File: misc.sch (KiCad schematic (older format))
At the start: 38 parts, among them J13 MICROSD_SLOT_TFP09-2-12B, P13 EXT_SD, P14 LCD, P15 LIMIT_SWITCHES, P16 LIMIT_SWITCHES_V, P17 CONN_01X03, P18 CONN_01X03, P19 CONN_01X03, P20 CONN_01X03, P21 THERMISTORS, P22 CONN_01X05, SW1 RESET, U2 24LC256

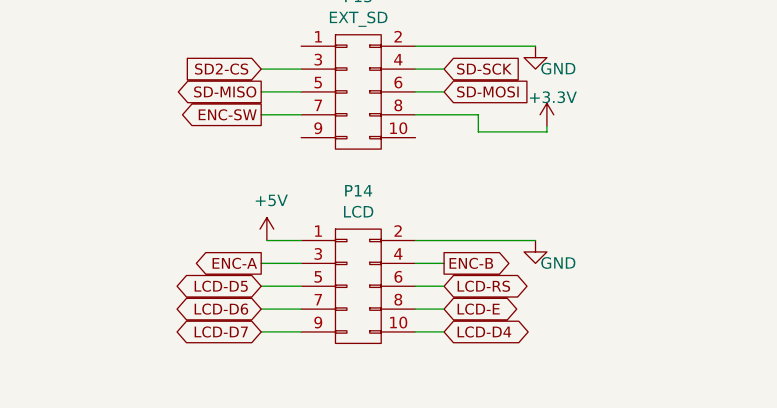
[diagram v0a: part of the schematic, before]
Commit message: More 3d stuff
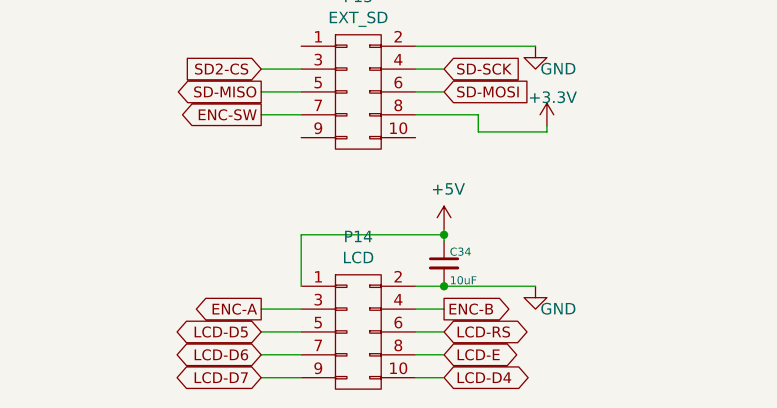
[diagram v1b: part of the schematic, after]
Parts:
- added C34: 10uF, Capacitors_SMD:C_0805, symbol C_Small
- P22: footprint geda-footprints:CON_HDR_1x5 -> armin-footprints:CON_HDR_1x5_2.54mm
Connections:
- net +5V: now also C34.1
- net GND: now also C34.2
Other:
- moved on the sheet: P14
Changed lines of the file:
@@
 SD-SCK
 $Comp
-L +3.3V #PWR083
+L +3.3V #PWR63
 U 1 1 568CFFAF
 P 1825 1775
-F 0 "#PWR083" H 1825 1625 50  0001 C CNN
+F 0 "#PWR63" H 1825 1625 50  0001 C CNN
 F 1 "+3.3V" H 1825 1925 35  0000 C CNN
 F 2 "" H 1825 1775 50  0000 C CNN
@@
 $EndComp
 $Comp
-L GND #PWR084
+L GND #PWR64
 U 1 1 568C59D5
 P 1825 1975
-F 0 "#PWR084" H 1825 1725 50  0001 C CNN
+F 0 "#PWR64" H 1825 1725 50  0001 C CNN
 F 1 "GND" H 1825 1825 35  0000 C CNN
 F 2 "" H 1825 1975 50  0000 C CNN
@@
 $EndComp
 $Comp
-L GND #PWR085
+L GND #PWR82
 U 1 1 568D834C
 P 9950 2075
-F 0 "#PWR085" H 9950 1825 50  0001 C CNN
+F 0 "#PWR82" H 9950 1825 50  0001 C CNN
 F 1 "GND" H 9958 1901 50  0000 C CNN
 F 2 "" H 9950 2075 50  0000 C CNN
@@
 $EndComp
 $Comp
-L GND #PWR086
+L GND #PWR81
 U 1 1 568D94E5
 P 8825 2325
-F 0 "#PWR086" H 8825 2075 50  0001 C CNN
+F 0 "#PWR81" H 8825 2075 50  0001 C CNN
 F 1 "GND" H 8833 2151 50  0000 C CNN
 F 2 "" H 8825 2325 50  0000 C CNN
@@
 $EndComp
 $Comp
-L +3V3 #PWR087
+L +3V3 #PWR80
 U 1 1 568D9512
 P 8825 1325
-F 0 "#PWR087" H 8825 1175 50  0001 C CNN
+F 0 "#PWR80" H 8825 1175 50  0001 C CNN
 F 1 "+3V3" H 8843 1499 50  0000 C CNN
 F 2 "" H 8825 1325 50  0000 C CNN
@@
 F 0 "P22" H 10527 1838 50  0000 L CNN
 F 1 "CONN_01X05" H 10527 1746 50  0000 L CNN
-F 2 "geda-footprints:CON_HDR_1x5" H 10450 1800 50  0001 C CNN
+F 2 "armin-footprints:CON_HDR_1x5_2.54mm" H 10450 1800 50  0001 C CNN
 F 3 "" H 10450 1800 50  0000 C CNN
 	1    10450 1800
@@
 $EndComp
 $Comp
-L +3V3 #PWR088
+L +3V3 #PWR83
 U 1 1 568D9A56
 P 10250 1525
-F 0 "#PWR088" H 10250 1375 50  0001 C CNN
+F 0 "#PWR83" H 10250 1375 50  0001 C CNN
 F 1 "+3V3" H 10268 1699 50  0000 C CNN
 F 2 "" H 10250 1525 50  0000 C CNN
@@
 $EndComp
 $Comp
-L GND #PWR089
+L GND #PWR67
 U 1 1 568DA443
 P 2875 3725
-F 0 "#PWR089" H 2875 3475 50  0001 C CNN
+F 0 "#PWR67" H 2875 3475 50  0001 C CNN
 F 1 "GND" H 2875 3575 50  0000 C CNN
 F 2 "" H 2875 3725 50  0000 C CNN
@@
 $EndComp
 $Comp
-L GND #PWR090
+L GND #PWR62
 U 1 1 568DA52A
 P 1775 4325
-F 0 "#PWR090" H 1775 4075 50  0001 C CNN
+F 0 "#PWR62" H 1775 4075 50  0001 C CNN
 F 1 "GND" H 1783 4151 50  0000 C CNN
 F 2 "" H 1775 4325 50  0000 C CNN
@@
 $EndComp
 $Comp
-L +3.3V #PWR091
+L +3.3V #PWR65
 U 1 1 568DA65A
 P 2175 3275
-F 0 "#PWR091" H 2175 3125 50  0001 C CNN
+F 0 "#PWR65" H 2175 3125 50  0001 C CNN
 F 1 "+3.3V" H 2193 3449 50  0000 C CNN
 F 2 "" H 2175 3275 50  0000 C CNN
@@
 $EndComp
 $Comp
-L GND #PWR092
+L GND #PWR76
 U 1 1 568D90A7
 P 6475 2225
-F 0 "#PWR092" H 6475 1975 50  0001 C CNN
+F 0 "#PWR76" H 6475 1975 50  0001 C CNN
 F 1 "GND" H 6483 2051 50  0000 C CNN
 F 2 "" H 6475 2225 50  0000 C CNN
@@
 $EndComp
 $Comp
-L +3.3V #PWR093
+L +3.3V #PWR77
 U 1 1 568D9133
 P 6900 1400
-F 0 "#PWR093" H 6900 1250 50  0001 C CNN
+F 0 "#PWR77" H 6900 1250 50  0001 C CNN
 F 1 "+3.3V" H 6918 1574 50  0000 C CNN
 F 2 "" H 6900 1400 50  0000 C CNN
@@
 $EndComp
 $Comp
-L GND #PWR094
+L GND #PWR74
 U 1 1 568DAACD
 P 5350 2375
-F 0 "#PWR094" H 5350 2125 50  0001 C CNN
+F 0 "#PWR74" H 5350 2125 50  0001 C CNN
 F 1 "GND" H 5358 2201 50  0000 C CNN
 F 2 "" H 5350 2375 50  0000 C CNN
@@
 $EndComp
 $Comp
-L +3.3V #PWR095
+L +3.3V #PWR68
 U 1 1 568E82EF
 P 3125 3600
-F 0 "#PWR095" H 3125 3450 50  0001 C CNN
+F 0 "#PWR68" H 3125 3450 50  0001 C CNN
 F 1 "+3.3V" H 3143 3774 50  0000 C CNN
 F 2 "" H 3125 3600 50  0000 C CNN
@@
 	7600 4550 7525 4550
 $Comp
-L GND #PWR096
+L GND #PWR78
 U 1 1 568EABC9
 P 7600 4800
-F 0 "#PWR096" H 7600 4550 50  0001 C CNN
+F 0 "#PWR78" H 7600 4550 50  0001 C CNN
 F 1 "GND" H 7608 4626 50  0000 C CNN
 F 2 "" H 7600 4800 50  0000 C CNN
@@
 $EndComp
 $Comp
-L +3.3V #PWR097
+L +3.3V #PWR79
 U 1 1 568EAEBC
 P 7675 2825
-F 0 "#PWR097" H 7675 2675 50  0001 C CNN
+F 0 "#PWR79" H 7675 2675 50  0001 C CNN
 F 1 "+3.3V" H 7693 2999 50  0000 C CNN
 F 2 "" H 7675 2825 50  0000 C CNN
@@
 L CONN_02X05 P14
 U 1 1 568EF014
-P 2400 6725
-F 0 "P14" H 2400 7141 50  0000 C CNN
-F 1 "LCD" H 2400 7049 50  0000 C CNN
-F 2 "armin-footprints:CON_HDR_2x5_2.54mm" H 2400 5525 50  0001 C CNN
-F 3 "" H 2400 5525 50  0000 C CNN
-	1    2400 6725
+P 2400 6925
+F 0 "P14" H 2400 7341 50  0000 C CNN
+F 1 "LCD" H 2400 7249 50  0000 C CNN
+F 2 "armin-footprints:CON_HDR_2x5_2.54mm" H 2400 5725 50  0001 C CNN
+F 3 "" H 2400 5725 50  0000 C CNN
+	1    2400 6925
 	1    0    0    -1
 $EndComp
@@
 SD-SCK
 $Comp
-L GND #PWR098
+L GND #PWR69
 U 1 1 568F027E
 P 3175 5675
-F 0 "#PWR098" H 3175 5425 50  0001 C CNN
+F 0 "#PWR69" H 3175 5425 50  0001 C CNN
 F 1 "GND" H 3275 5575 50  0000 C CNN
 F 2 "" H 3175 5675 50  0000 C CNN
@@
 	2650 5675 3175 5675
 $Comp
-L +3.3V #PWR099
+L +3.3V #PWR71
 U 1 1 568F1103
 P 3225 6025
-F 0 "#PWR099" H 3225 5875 50  0001 C CNN
+F 0 "#PWR71" H 3225 5875 50  0001 C CNN
 F 1 "+3.3V" H 3250 6150 50  0000 C CNN
 F 2 "" H 3225 6025 50  0000 C CNN
@@
 	3225 6050 3225 6025
 $Comp
-L +5V #PWR0100
+L +5V #PWR66
 U 1 1 568F17B3
-P 2000 6525
-F 0 "#PWR0100" H 2000 6375 50  0001 C CNN
-F 1 "+5V" H 2018 6699 50  0000 C CNN
-F 2 "" H 2000 6525 50  0000 C CNN
-F 3 "" H 2000 6525 50  0000 C CNN
-	1    2000 6525
-	1    0    0    -1
-$EndComp
-$Comp
-L GND #PWR0101
+P 2775 6475
+F 0 "#PWR66" H 2775 6325 50  0001 C CNN
+F 1 "+5V" H 2793 6649 50  0000 C CNN
+F 2 "" H 2775 6475 50  0000 C CNN
+F 3 "" H 2775 6475 50  0000 C CNN
+	1    2775 6475
+	1    0    0    -1
+$EndComp
+$Comp
+L GND #PWR70
 U 1 1 568F18BA
-P 3175 6525
-F 0 "#PWR0101" H 3175 6275 50  0001 C CNN
-F 1 "GND" H 3275 6425 50  0000 C CNN
-F 2 "" H 3175 6525 50  0000 C CNN
-F 3 "" H 3175 6525 50  0000 C CNN
-	1    3175 6525
-	1    0    0    -1
-$EndComp
-Wire Wire Line
-	2650 6525 3175 6525
-Wire Wire Line
-	2000 6525 2150 6525
-Text GLabel 1975 6625 0    47   Output ~ 0
+P 3175 6725
+F 0 "#PWR70" H 3175 6475 50  0001 C CNN
+F 1 "GND" H 3275 6625 50  0000 C CNN
+F 2 "" H 3175 6725 50  0000 C CNN
+F 3 "" H 3175 6725 50  0000 C CNN
+	1    3175 6725
+	1    0    0    -1
+$EndComp
+Wire Wire Line
+	2650 6725 3175 6725
+Text GLabel 1975 6825 0    47   Output ~ 0
 ENC-A
-Text GLabel 2775 6625 2    47   Output ~ 0
+Text GLabel 2775 6825 2    47   Output ~ 0
 ENC-B
 Wire Wire Line
-	2650 6625 2775 6625
-Wire Wire Line
-	2150 6625 1975 6625
-Text GLabel 1975 6725 0    47   BiDi ~ 0
+	2650 6825 2775 6825
+Wire Wire Line
+	2150 6825 1975 6825
+Text GLabel 1975 6925 0    47   BiDi ~ 0
 LCD-D5
-Text GLabel 1975 6825 0    47   BiDi ~ 0
+Text GLabel 1975 7025 0    47   BiDi ~ 0
 LCD-D6
-Text GLabel 1975 6925 0    47   BiDi ~ 0
+Text GLabel 1975 7125 0    47   BiDi ~ 0
 LCD-D7
+Text GLabel 2775 7125 2    47   BiDi ~ 0
+LCD-D4
+Text GLabel 2775 7025 2    47   BiDi ~ 0
+LCD-E
 Text GLabel 2775 6925 2    47   BiDi ~ 0
-LCD-D4
-Text GLabel 2775 6825 2    47   BiDi ~ 0
-LCD-E
-Text GLabel 2775 6725 2    47   BiDi ~ 0
 LCD-RS
 Wire Wire Line
-	1975 6725 2150 6725
-Wire Wire Line
-	2150 6825 1975 6825
-Wire Wire Line
 	1975 6925 2150 6925
 Wire Wire Line
-	2650 6725 2775 6725
-Wire Wire Line
-	2775 6825 2650 6825
+	2150 7025 1975 7025
+Wire Wire Line
+	1975 7125 2150 7125
 Wire Wire Line
 	2650 6925 2775 6925
+Wire Wire Line
+	2775 7025 2650 7025
+Wire Wire Line
+	2650 7125 2775 7125
 Text GLabel 8250 1600 0    47   Output ~ 0
 T0
@@
 	5325 4225 5325 4200
 $Comp
-L +3.3V #PWR0102
+L +3.3V #PWR72
 U 1 1 568F9643
 P 5325 3575
-F 0 "#PWR0102" H 5325 3425 50  0001 C CNN
+F 0 "#PWR72" H 5325 3425 50  0001 C CNN
 F 1 "+3.3V" H 5343 3749 50  0000 C CNN
 F 2 "" H 5325 3575 50  0000 C CNN
@@
 	4900 4950 5050 4950
 $Comp
-L GND #PWR0103
+L GND #PWR73
 U 1 1 568F9E88
 P 5325 5350
-F 0 "#PWR0103" H 5325 5100 50  0001 C CNN
+F 0 "#PWR73" H 5325 5100 50  0001 C CNN
 F 1 "GND" H 5333 5176 50  0000 C CNN
 F 2 "" H 5325 5350 50  0000 C CNN
@@
 $EndComp
 $Comp
-L +3.3V #PWR0104
+L +3.3V #PWR75
 U 1 1 56944144
 P 6475 1275
-F 0 "#PWR0104" H 6475 1125 50  0001 C CNN
+F 0 "#PWR75" H 6475 1125 50  0001 C CNN
 F 1 "+3.3V" H 6493 1449 50  0000 C CNN
 F 2 "" H 6475 1275 50  0000 C CNN
@@
 	6475 1275 6475 1325
 Connection ~ 5325 5350
+$Comp
+L C_Small C34
+U 1 1 56976953
+P 2775 6625
+F 0 "C34" H 2800 6675 35  0000 L CNN
+F 1 "10uF" H 2800 6550 35  0000 L CNN
+F 2 "Capacitors_SMD:C_0805" H 2775 6625 50  0001 C CNN
+F 3 "" H 2775 6625 50  0000 C CNN
+	1    2775 6625
+	1    0    0    -1
+$EndComp
+Wire Wire Line
+	2775 6475 2775 6525
+Wire Wire Line
+	2775 6500 2150 6500
+Wire Wire Line
+	2150 6500 2150 6725
+Connection ~ 2775 6500
+Connection ~ 2775 6725
 $EndSCHEMATC

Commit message: More 3d stuff
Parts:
- C18, C26, C27, C28, C29, C30, C33, C34: footprint Capacitors_SMD:C_0805 -> capacitors:C_0805
- C19, C20, C21, C22, C23, C24, C25, C31, C32: footprint Capacitors_SMD:C_0603 -> capacitors:C_0603
- D17: footprint armin-footprints:0603diode -> diodes:LED-0603
- R35, R36, R37, R38, R39, R40, R41, R42: footprint Resistors_SMD:R_0603 -> resistors:R_0603
- U2: footprint armin-footprints:SOIC8 -> soic:SOIC8
